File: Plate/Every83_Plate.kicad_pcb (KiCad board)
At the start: 2 copper layers, 333.6 x 134 mm, 84 parts

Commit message: update the plate dimensions
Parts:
- removed REF**: DFR0995_Mounting_holes, JohnDeereLibrary:DFR0995_Mounting_holes
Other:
- board size 333.6 x 134 mm -> 331.6 x 134 mm

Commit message: change plate mounting style
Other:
- board size 331.6 x 134 mm -> 331.6 x 133.7 mm

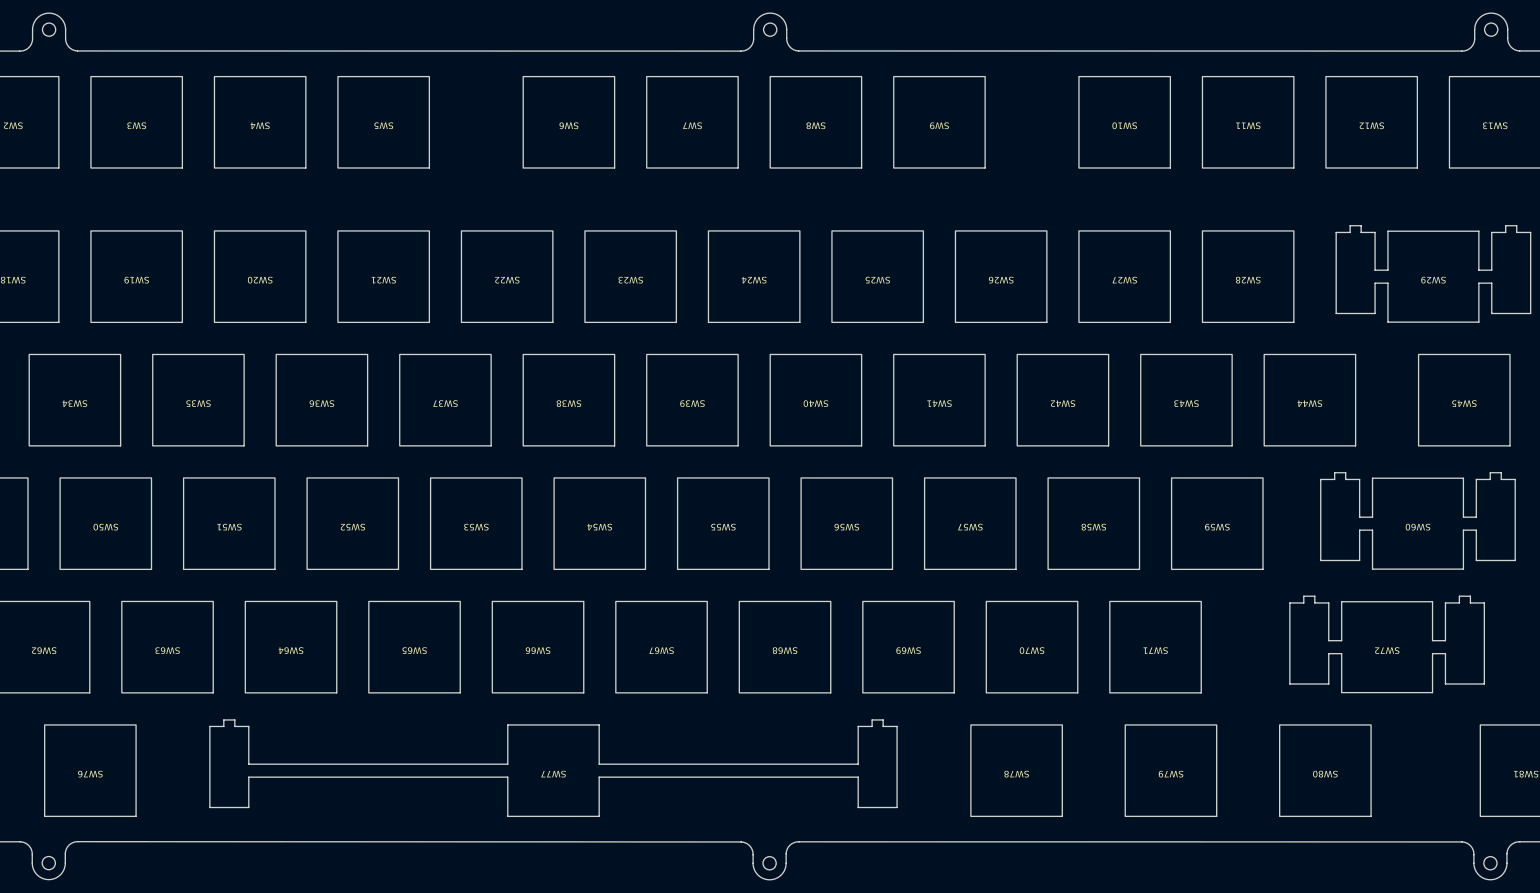
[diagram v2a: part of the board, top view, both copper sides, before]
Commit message: small changes
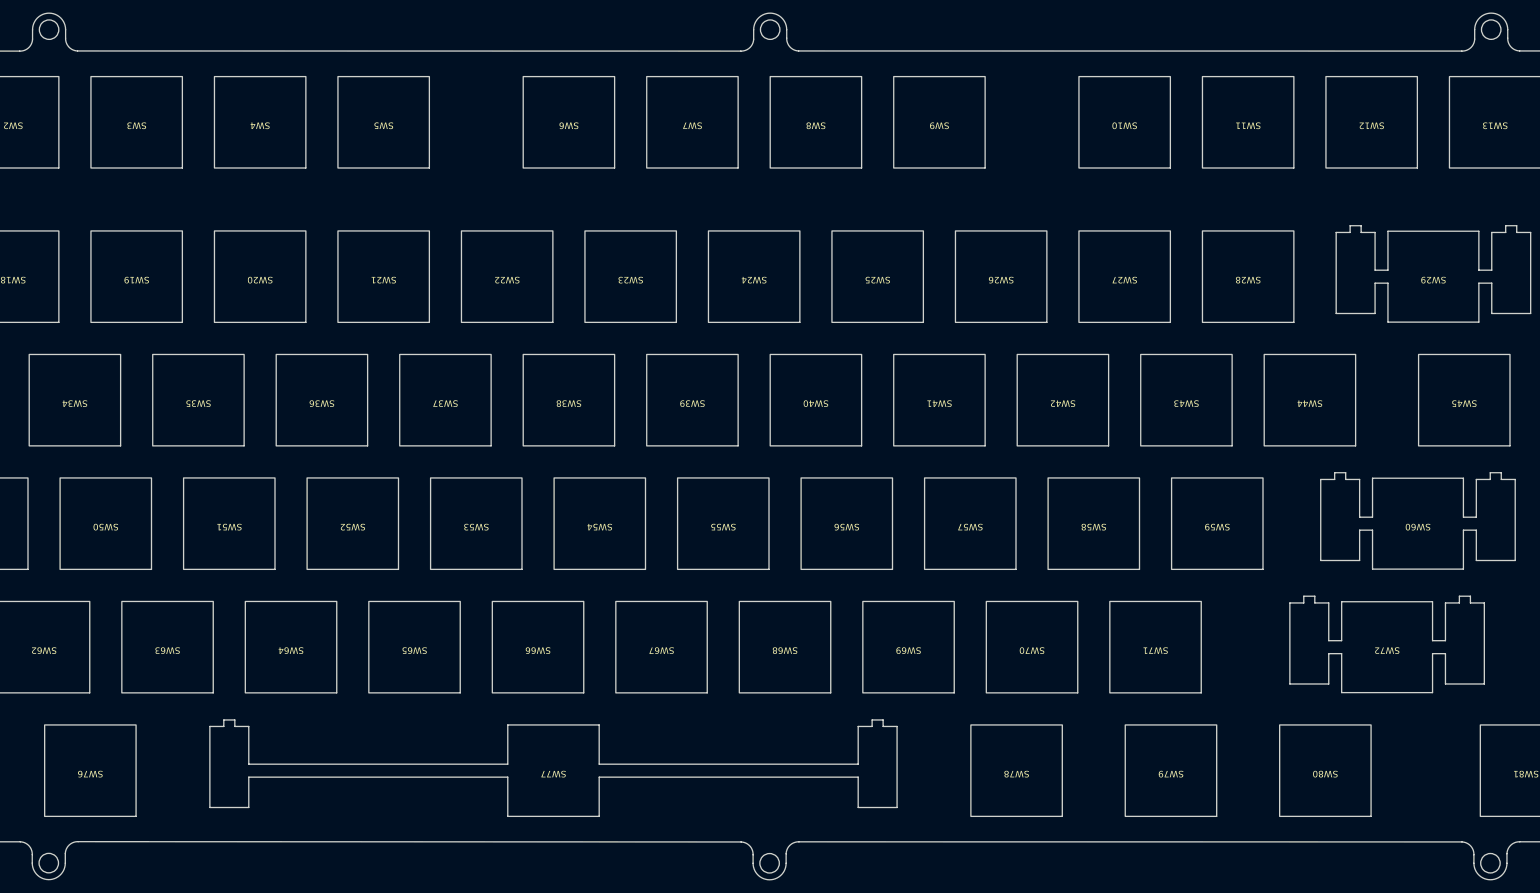
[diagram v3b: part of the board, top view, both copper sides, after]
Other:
- outline, holes or cut-outs redrawn
